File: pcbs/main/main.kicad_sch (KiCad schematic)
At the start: 14 parts

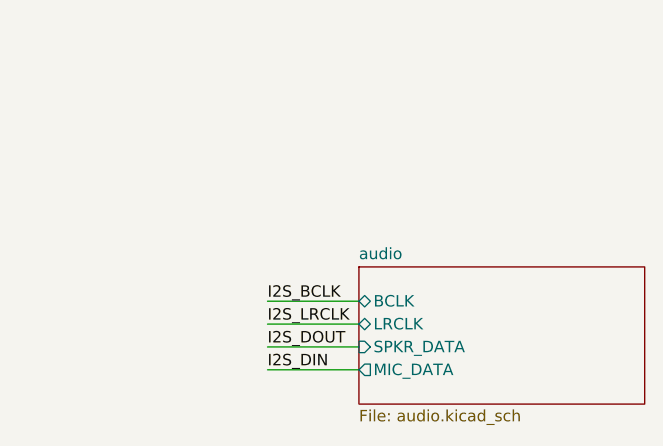
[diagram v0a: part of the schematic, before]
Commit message: Add microphone ADC
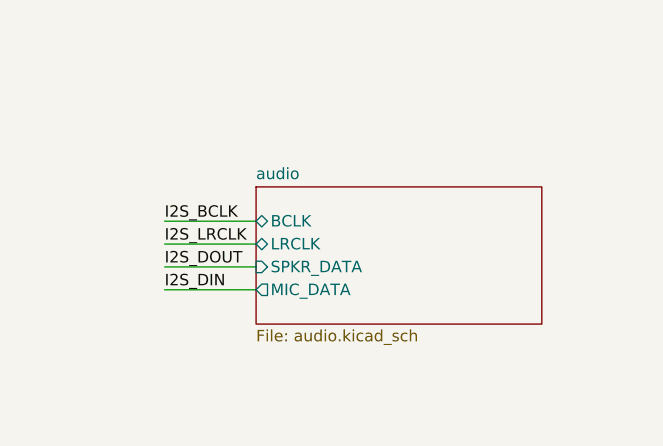
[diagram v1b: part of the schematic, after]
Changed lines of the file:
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@@
     (stroke (width 0) (type default) (color 0 0 0 0))
   )
-  (wire (pts (xy 124.46 179.07) (xy 134.62 179.07))
+  (wire (pts (xy 113.03 170.18) (xy 123.19 170.18))
     (stroke (width 0) (type default) (color 0 0 0 0))
   )
@@
     (stroke (width 0) (type default) (color 0 0 0 0))
   )
-  (wire (pts (xy 124.46 176.53) (xy 134.62 176.53))
+  (wire (pts (xy 113.03 167.64) (xy 123.19 167.64))
     (stroke (width 0) (type default) (color 0 0 0 0))
   )
@@
     (stroke (width 0) (type default) (color 0 0 0 0))
   )
-  (wire (pts (xy 124.46 181.61) (xy 134.62 181.61))
+  (wire (pts (xy 113.03 172.72) (xy 123.19 172.72))
     (stroke (width 0) (type default) (color 0 0 0 0))
   )
@@
     (stroke (width 0) (type default) (color 0 0 0 0))
   )
-  (wire (pts (xy 124.46 184.15) (xy 134.62 184.15))
+  (wire (pts (xy 113.03 175.26) (xy 123.19 175.26))
     (stroke (width 0) (type default) (color 0 0 0 0))
   )
@@
     (effects (font (size 1.27 1.27)) (justify left bottom))
   )
-  (label "I2S_DIN" (at 124.46 184.15 0)
+  (label "I2S_DIN" (at 113.03 175.26 0)
     (effects (font (size 1.27 1.27)) (justify left bottom))
   )
@@
     (effects (font (size 1.27 1.27)) (justify left bottom))
   )
-  (label "I2S_BCLK" (at 124.46 176.53 0)
+  (label "I2S_BCLK" (at 113.03 167.64 0)
     (effects (font (size 1.27 1.27)) (justify left bottom))
   )
-  (label "I2S_LRCLK" (at 124.46 179.07 0)
+  (label "I2S_LRCLK" (at 113.03 170.18 0)
     (effects (font (size 1.27 1.27)) (justify left bottom))
   )
-  (label "I2S_DOUT" (at 124.46 181.61 0)
+  (label "I2S_DOUT" (at 113.03 172.72 0)
     (effects (font (size 1.27 1.27)) (justify left bottom))
   )
@@
     (pin "2")
   )
-  (sheet (at 134.62 172.72) (size 31.75 15.24) (fields_autoplaced)
+  (sheet (at 123.19 163.83) (size 31.75 15.24) (fields_autoplaced)
     (stroke (width 0.1524) (type solid) (color 0 0 0 0))
     (fill (color 0 0 0 0.0000))
-    (property "Sheet name" "audio" (id 0) (at 134.62 172.0084 0)
+    (property "Sheet name" "audio" (id 0) (at 123.19 163.1184 0)
       (effects (font (size 1.27 1.27)) (justify left bottom))
     )
-    (property "Sheet file" "audio.kicad_sch" (id 1) (at 134.62 188.5446 0)
+    (property "Sheet file" "audio.kicad_sch" (id 1) (at 123.19 179.6546 0)
       (effects (font (size 1.27 1.27)) (justify left top))
     )
-    (pin "MIC_DATA" output (at 134.62 184.15 180)
-      (effects (font (size 1.27 1.27)) (justify left))
-    )
-    (pin "BCLK" bidirectional (at 134.62 176.53 180)
-      (effects (font (size 1.27 1.27)) (justify left))
-    )
-    (pin "SPKR_DATA" input (at 134.62 181.61 180)
-      (effects (font (size 1.27 1.27)) (justify left))
-    )
-    (pin "LRCLK" bidirectional (at 134.62 179.07 180)
+    (pin "MIC_DATA" output (at 123.19 175.26 180)
+      (effects (font (size 1.27 1.27)) (justify left))
+    )
+    (pin "BCLK" bidirectional (at 123.19 167.64 180)
+      (effects (font (size 1.27 1.27)) (justify left))
+    )
+    (pin "SPKR_DATA" input (at 123.19 172.72 180)
+      (effects (font (size 1.27 1.27)) (justify left))
+    )
+    (pin "LRCLK" bidirectional (at 123.19 170.18 180)
       (effects (font (size 1.27 1.27)) (justify left))
     )
@@
       (reference "#PWR?") (unit 1) (value "GND") (footprint "")
     )
+    (path "/c9bcbb20-bce5-48eb-aaa8-469331798139/46cc0fd6-5127-4541-8cbd-16b3c454ec30"
+      (reference "#PWR?") (unit 1) (value "+3V3") (footprint "")
+    )
+    (path "/c9bcbb20-bce5-48eb-aaa8-469331798139/49c576fb-36cc-457c-913f-64856c713747"
+      (reference "#PWR?") (unit 1) (value "GND") (footprint "")
+    )
+    (path "/c9bcbb20-bce5-48eb-aaa8-469331798139/51180f80-2e38-4b4b-bcae-d935a452b9ac"
+      (reference "#PWR?") (unit 1) (value "GND") (footprint "")
+    )
     (path "/5a3e5c1e-d818-454f-996c-fc29d038aef8"
       (reference "#PWR?") (unit 1) (value "+3V3") (footprint "")
@@
     )
     (path "/60e34a1e-e74b-4478-a63b-76a18bae9efe"
+      (reference "#PWR?") (unit 1) (value "GND") (footprint "")
+    )
+    (path "/c9bcbb20-bce5-48eb-aaa8-469331798139/66e41d15-58fe-421c-879c-5a5ec35cc159"
+      (reference "#PWR?") (unit 1) (value "GND") (footprint "")
+    )
+    (path "/c9bcbb20-bce5-48eb-aaa8-469331798139/73507f45-6922-46a3-97fd-24e7efed8d39"
+      (reference "#PWR?") (unit 1) (value "GND") (footprint "")
+    )
+    (path "/c9bcbb20-bce5-48eb-aaa8-469331798139/7c325a6b-c170-4c02-9aea-34e929f042b3"
       (reference "#PWR?") (unit 1) (value "GND") (footprint "")
     )
@@
       (reference "#PWR?") (unit 1) (value "+3V3") (footprint "")
     )
+    (path "/c9bcbb20-bce5-48eb-aaa8-469331798139/e8bcc4b4-c48e-4987-a93f-f4bd0390d3d4"
+      (reference "#PWR?") (unit 1) (value "GND") (footprint "")
+    )
+    (path "/c9bcbb20-bce5-48eb-aaa8-469331798139/eaa9c740-0990-484c-9f57-70927834192b"
+      (reference "#PWR?") (unit 1) (value "+3V3") (footprint "")
+    )
+    (path "/c9bcbb20-bce5-48eb-aaa8-469331798139/eda44fcb-6711-4f46-a108-b2fd9ef9a41d"
+      (reference "#PWR?") (unit 1) (value "+3V3") (footprint "")
+    )
+    (path "/c9bcbb20-bce5-48eb-aaa8-469331798139/fe60cf0c-f0d7-41ae-8957-bf23b0dc3dec"
+      (reference "#PWR?") (unit 1) (value "GND") (footprint "")
+    )
     (path "/09a2e506-7b9e-4939-b88b-3d561d5c8ab0"
       (reference "C?") (unit 1) (value "10n") (footprint "")
@@
       (reference "C?") (unit 1) (value "10u") (footprint "")
     )
+    (path "/c9bcbb20-bce5-48eb-aaa8-469331798139/1740d004-8130-497a-b9db-37a01a9a22ca"
+      (reference "C?") (unit 1) (value "10u") (footprint "")
+    )
     (path "/c9bcbb20-bce5-48eb-aaa8-469331798139/2fecbd38-48ed-441e-8503-3637d2228528"
       (reference "C?") (unit 1) (value "220u") (footprint "")
     )
+    (path "/c9bcbb20-bce5-48eb-aaa8-469331798139/37c30413-4384-47d2-a5e4-0116e2e37447"
+      (reference "C?") (unit 1) (value "10u") (footprint "")
+    )
     (path "/c9bcbb20-bce5-48eb-aaa8-469331798139/4be6c124-ae67-4a93-92c3-f5ebb66896d2"
       (reference "C?") (unit 1) (value "10u") (footprint "")
@@
       (reference "C?") (unit 1) (value "0.05u") (footprint "")
     )
+    (path "/c9bcbb20-bce5-48eb-aaa8-469331798139/5d70e13c-3030-4e6c-83a4-db0b7b040848"
+      (reference "C?") (unit 1) (value "0.1u") (footprint "")
+    )
+    (path "/c9bcbb20-bce5-48eb-aaa8-469331798139/6693416e-c218-4225-bf8c-203de3184cc6"
+      (reference "C?") (unit 1) (value "0.1u") (footprint "")
+    )
     (path "/c9bcbb20-bce5-48eb-aaa8-469331798139/6d17e313-32c7-43d0-b4c7-349c774d30c7"
       (reference "C?") (unit 1) (value "2.2n") (footprint "")
     )
+    (path "/c9bcbb20-bce5-48eb-aaa8-469331798139/83b9a4f1-f335-4bc2-9cad-cc27bdf156a7"
+      (reference "C?") (unit 1) (value "2.2u") (footprint "")
+    )
     (path "/c9bcbb20-bce5-48eb-aaa8-469331798139/8d8d8faf-6c60-404a-ab82-3bfacff52694"
       (reference "C?") (unit 1) (value "0.1u") (footprint "")
@@
       (reference "C?") (unit 1) (value "2.2u") (footprint "")
     )
+    (path "/c9bcbb20-bce5-48eb-aaa8-469331798139/a3942f56-db20-4420-a986-eb6c91fb6e06"
+      (reference "C?") (unit 1) (value "0.1u") (footprint "")
+    )
     (path "/c9bcbb20-bce5-48eb-aaa8-469331798139/b5d0444e-9218-4252-8254-6ae7f6e3ab2b"
       (reference "C?") (unit 1) (value "10u") (footprint "")
     )
+    (path "/c9bcbb20-bce5-48eb-aaa8-469331798139/b788ad77-918e-4172-89e1-a03585ef8812"
+      (reference "C?") (unit 1) (value "0.1u") (footprint "")
+    )
     (path "/c9bcbb20-bce5-48eb-aaa8-469331798139/ba7673e9-d14c-42cd-b620-ecb3145f737a"
+      (reference "C?") (unit 1) (value "10u") (footprint "")
+    )
+    (path "/c9bcbb20-bce5-48eb-aaa8-469331798139/bebccbaf-f974-4003-b23e-0cb0ed3ca32a"
       (reference "C?") (unit 1) (value "10u") (footprint "")
     )
@@
       (reference "C?") (unit 1) (value "100u") (footprint "")
     )
+    (path "/c9bcbb20-bce5-48eb-aaa8-469331798139/f37ff452-6805-4d29-95dc-80fe3ff7b009"
+      (reference "C?") (unit 1) (value "10u") (footprint "")
+    )
     (path "/c9bcbb20-bce5-48eb-aaa8-469331798139/f4736beb-955e-45d9-bb04-c50f6218e7c1"
       (reference "C?") (unit 1) (value "2.2u") (footprint "")
     )
+    (path "/c9bcbb20-bce5-48eb-aaa8-469331798139/f8d60052-1827-4f0b-b9d5-716c323a0d62"
+      (reference "C?") (unit 1) (value "10u") (footprint "")
+    )
     (path "/c9bcbb20-bce5-48eb-aaa8-469331798139/fac9f493-6f0a-4587-9630-d6aa4c9b4397"
       (reference "C?") (unit 1) (value "100u") (footprint "")
@@
       (reference "LS?") (unit 1) (value "Speaker") (footprint "")
     )
+    (path "/c9bcbb20-bce5-48eb-aaa8-469331798139/f6a63bdb-a497-4bdc-b614-039d74749a43"
+      (reference "MK?") (unit 1) (value "Microphone") (footprint "")
+    )
     (path "/c9bcbb20-bce5-48eb-aaa8-469331798139/165ee7e1-b0f3-41a6-818b-678b0c672594"
       (reference "R?") (unit 1) (value "10k") (footprint "")
@@
       (reference "R?") (unit 1) (value "R") (footprint "")
     )
+    (path "/c9bcbb20-bce5-48eb-aaa8-469331798139/f8ee2805-625c-4280-b190-8aec0c73cf9b"
+      (reference "R?") (unit 1) (value "2k2") (footprint "")
+    )
     (path "/c9bcbb20-bce5-48eb-aaa8-469331798139/0c820c07-8709-47be-8e45-880d1b3be58e"
       (reference "U?") (unit 1) (value "LM386N-4") (footprint "")
@@
       (reference "U?") (unit 1) (value "CAT24C32") (footprint "")
     )
-    (path "/c9bcbb20-bce5-48eb-aaa8-469331798139/15d0d989-c057-47ce-a42b-bc0875b50f04"
-      (reference "U?") (unit 1) (value "AK5720VT") (footprint "Package_SO:TSSOP-16_4.4x5mm_P0.65mm")
+    (path "/c9bcbb20-bce5-48eb-aaa8-469331798139/8e331940-2b25-4cb2-b301-bce402d550e1"
+      (reference "U?") (unit 1) (value "PCM1860") (footprint "")
     )
     (path "/a4557600-a8ae-411b-b0f5-d7b885f9c0f1"
